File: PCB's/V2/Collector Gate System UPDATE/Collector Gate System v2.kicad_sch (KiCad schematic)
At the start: 30 parts, among them J1 24Vac, Sw1 Screw_Terminal_01x02, Sw2 Screw_Terminal_01x02, Sw3 Screw_Terminal_01x02, Sw4 Screw_Terminal_01x02, U1 LM7805_TO220, U2 MC33063AD

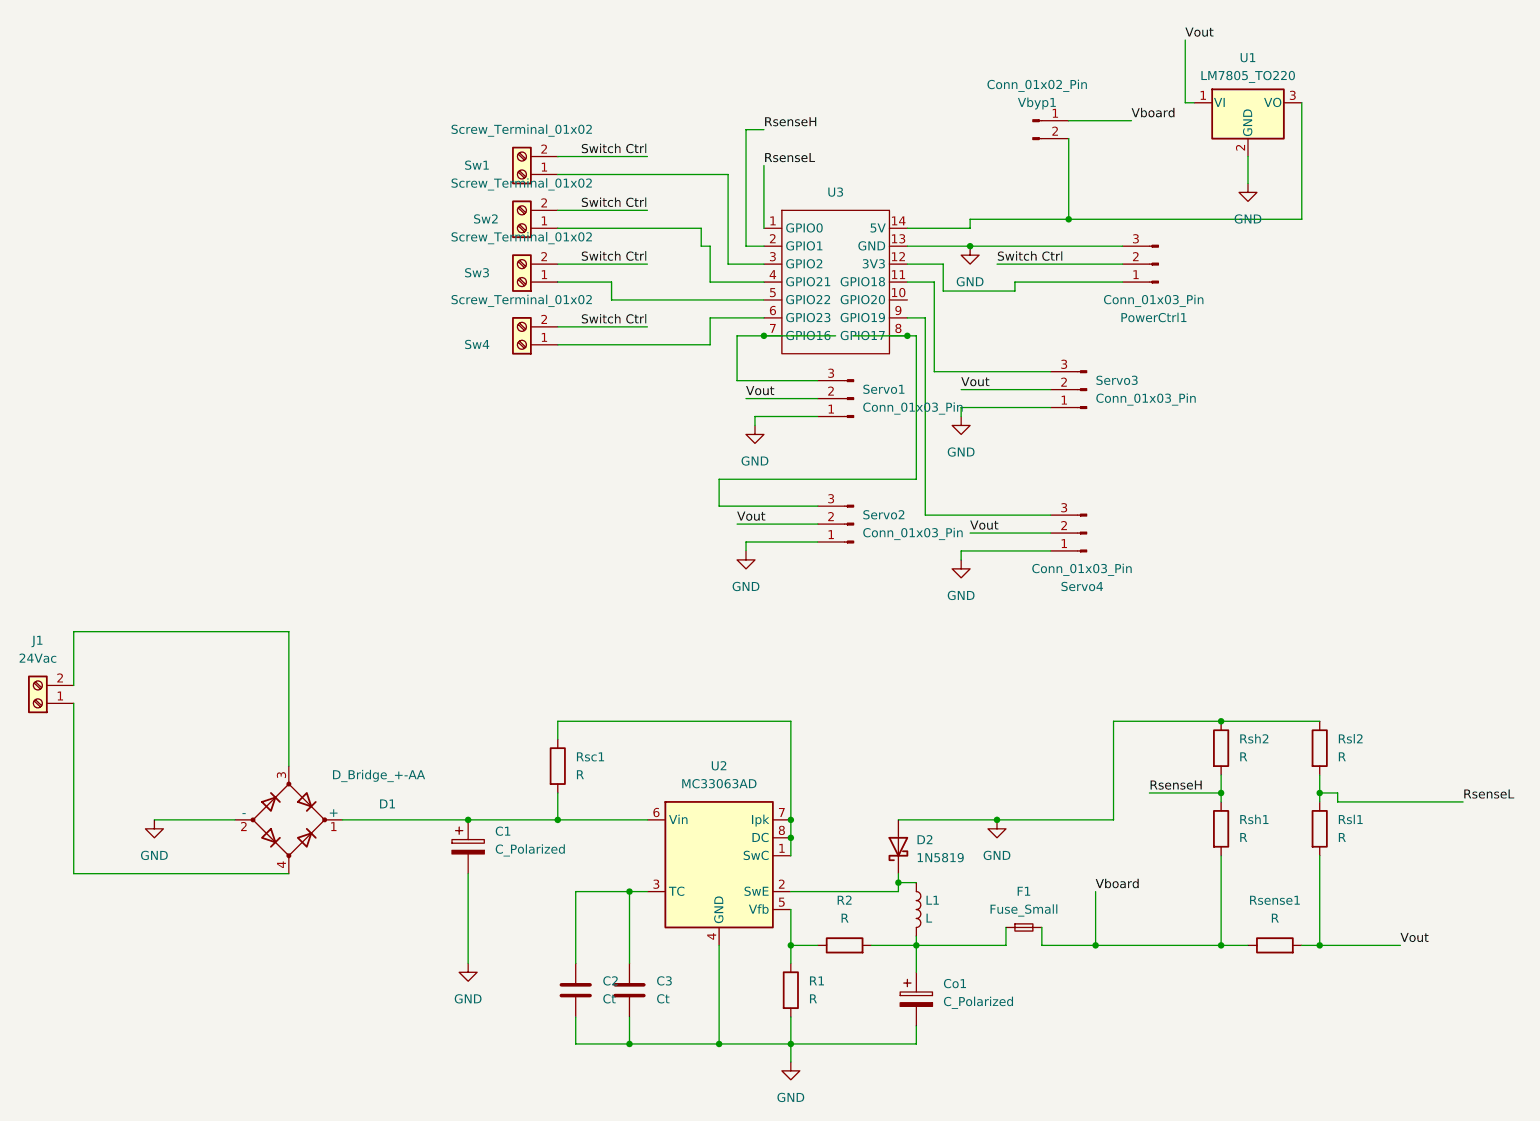
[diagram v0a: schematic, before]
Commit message: load
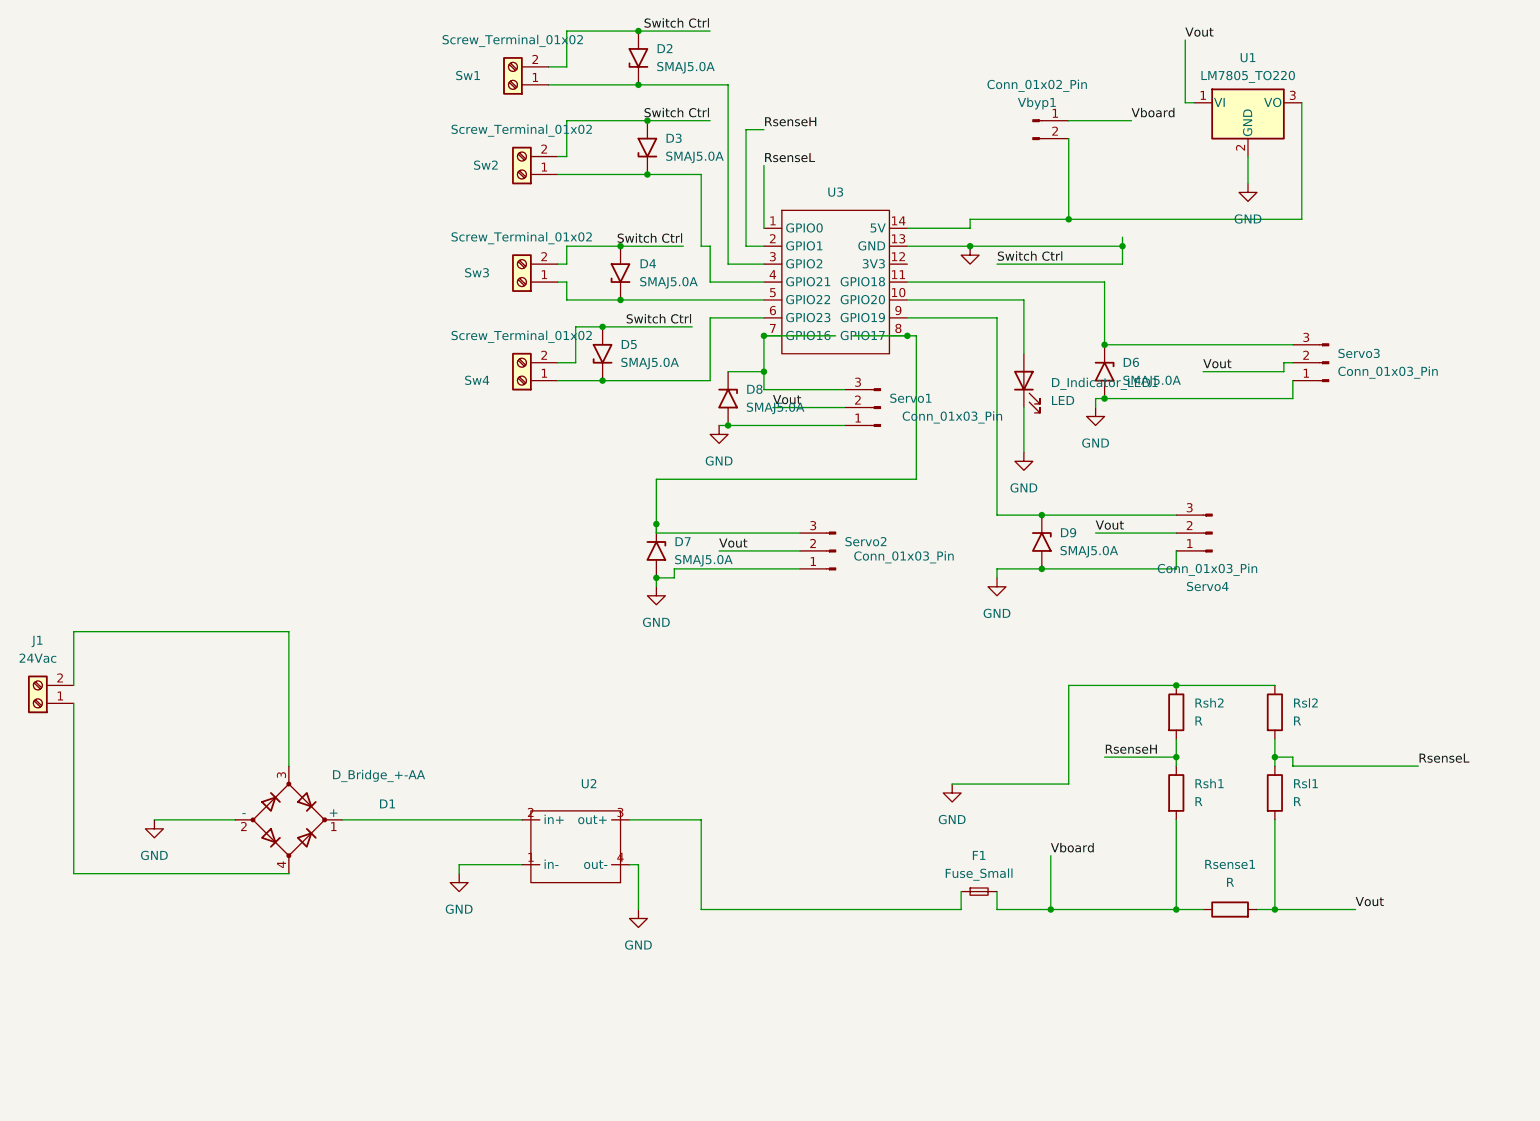
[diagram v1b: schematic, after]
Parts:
- removed C1: C_Polarized, Capacitor_THT:CP_Radial_D8.0mm_P2.50mm, symbol Device:C_Polarized
- removed C2: Ct, Capacitor_SMD:C_0603_1608Metric_Pad1.08x0.95mm_HandSolder, symbol Device:C
- removed C3: Ct, Capacitor_THT:C_Rect_L4.0mm_W2.5mm_P2.50mm, symbol Device:C
- removed Co1: C_Polarized, Capacitor_THT:CP_Radial_D8.0mm_P3.80mm, symbol Device:C_Polarized
- removed D2: 1N5819, Diode_THT:D_DO-41_SOD81_P10.16mm_Horizontal, symbol Diode:1N5819
- removed L1: L, Inductor_THT:L_Axial_L16.0mm_D7.5mm_P7.62mm_Vertical_Fastron_XHBCC, symbol Device:L
- removed PowerCtrl1: Conn_01x03_Pin, Connector_PinHeader_2.54mm:PinHeader_1x03_P2.54mm_Vertical, symbol Connector:Conn_01x03_Pin
- removed R1, R2: R, Resistor_THT:R_Axial_DIN0207_L6.3mm_D2.5mm_P10.16mm_Horizontal, symbol Device:R
- removed Rsc1: R, Resistor_THT:R_Axial_DIN0411_L9.9mm_D3.6mm_P12.70mm_Horizontal, symbol Device:R
- removed U2: MC33063AD, Package_SO:SOIC-8_3.9x4.9mm_P1.27mm, symbol Regulator_Switching:MC33063AD
- added D2, D3, D4, D5, D6, D7, D8, D9: SMAJ5.0A, Diode_SMD:D_SMA, symbol Diode:SMAJ5.0A
- added D_Indicator_LED1: LED, LED_THT:LED_D5.0mm_Clear, symbol Device:LED
- added U2: ~, CustomParts:MS1584_fullboard, symbol Custom_PArts:MP1584_Fullboard
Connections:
- net Switch Ctrl is gone; now on net GND: Sw1.2 (Pin_2), Sw2.2 (Pin_2), Sw3.2 (Pin_2), Sw4.2 (Pin_2)
- net GND: now also D2.2 (A2), D3.2 (A2), D4.2 (A2), D5.2 (A2), D6.2 (A2), D7.2 (A2), D8.2 (A2), D9.2 (A2), D_Indicator_LED1.1 (K), U2.1 (in-), U2.4 (out-)
- net at Sw1.1 (Pin_1), U3.3 (GPIO2): now also D2.1 (A1)
- net at D1.1 (+): now also U2.2 (in+)
- net at Servo3.3 (Pin_3), U3.11 (GPIO18): now also D6.1 (A1)
- net at Servo2.3 (Pin_3), U3.8 (GPIO17): now also D7.1 (A1)
- net at Servo4.3 (Pin_3), U3.9 (GPIO19): now also D9.1 (A1)
- net at F1.1: now also U2.3 (out+)
- net at Servo1.3 (Pin_3), U3.7 (GPIO16): now also D8.1 (A1)
- net at Sw3.1 (Pin_1), U3.5 (GPIO22): now also D4.1 (A1)
- net at Sw2.1 (Pin_1), U3.4 (GPIO21): now also D3.1 (A1)
- net at U3.10 (GPIO20): now also D_Indicator_LED1.2 (A)
- net at Sw4.1 (Pin_1), U3.6 (GPIO23): now also D5.1 (A1)
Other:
- moved on the sheet: Rsense1, Rsh1, Rsh2, Rsl1, Rsl2, Servo1, Servo2, Servo3, Servo4, Sw1, Sw2, Sw4
